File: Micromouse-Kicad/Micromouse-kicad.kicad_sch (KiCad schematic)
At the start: 101 parts, among them J1 SWD, J2 USB_B_Micro, J3 UARTBTH, J4 Batería, J5 VL6180x, J6 MotorEncodL, J7 MotorEncodR, Q1 BS170, Q2 BS170, Q3 BS170, Q4 BS170, SW1 RST, SW2 BootSwitch, SW3 PowerSwitch, SW4 BTN, SW5 BTN, U1 STM32F405RGT6, U10 TCRT5000, U2 AMS1117-5.0, U3 AMS1117-3.3, U4 SRV05-4, U5 MPU-6500, U6 DRV8833PWPR, U7 TCRT5000, U8 TCRT5000, U9 TCRT5000, Y1 8MHz

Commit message: Casi todo routeado
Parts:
- R4: footprint Resistor_SMD:R_0402_1005Metric -> Resistor_SMD:R_0603_1608Metric
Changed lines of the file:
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@@
       (effects (font (size 1.27 1.27)) (justify left))
     )
-    (property "Footprint" "Resistor_SMD:R_0402_1005Metric" (id 2) (at 165.1 157.48 0)
+    (property "Footprint" "Resistor_SMD:R_0603_1608Metric" (id 2) (at 165.1 157.48 0)
       (effects (font (size 1.27 1.27)) hide)
     )
@@
     )
     (path "/45c613f9-aec8-424a-b480-e2cd3c7f1c41"
-      (reference "R4") (unit 1) (value "220") (footprint "Resistor_SMD:R_0402_1005Metric")
+      (reference "R4") (unit 1) (value "220") (footprint "Resistor_SMD:R_0603_1608Metric")
     )
     (path "/3e5cccc0-5e8e-4d7a-84ba-3564961b6bdd"

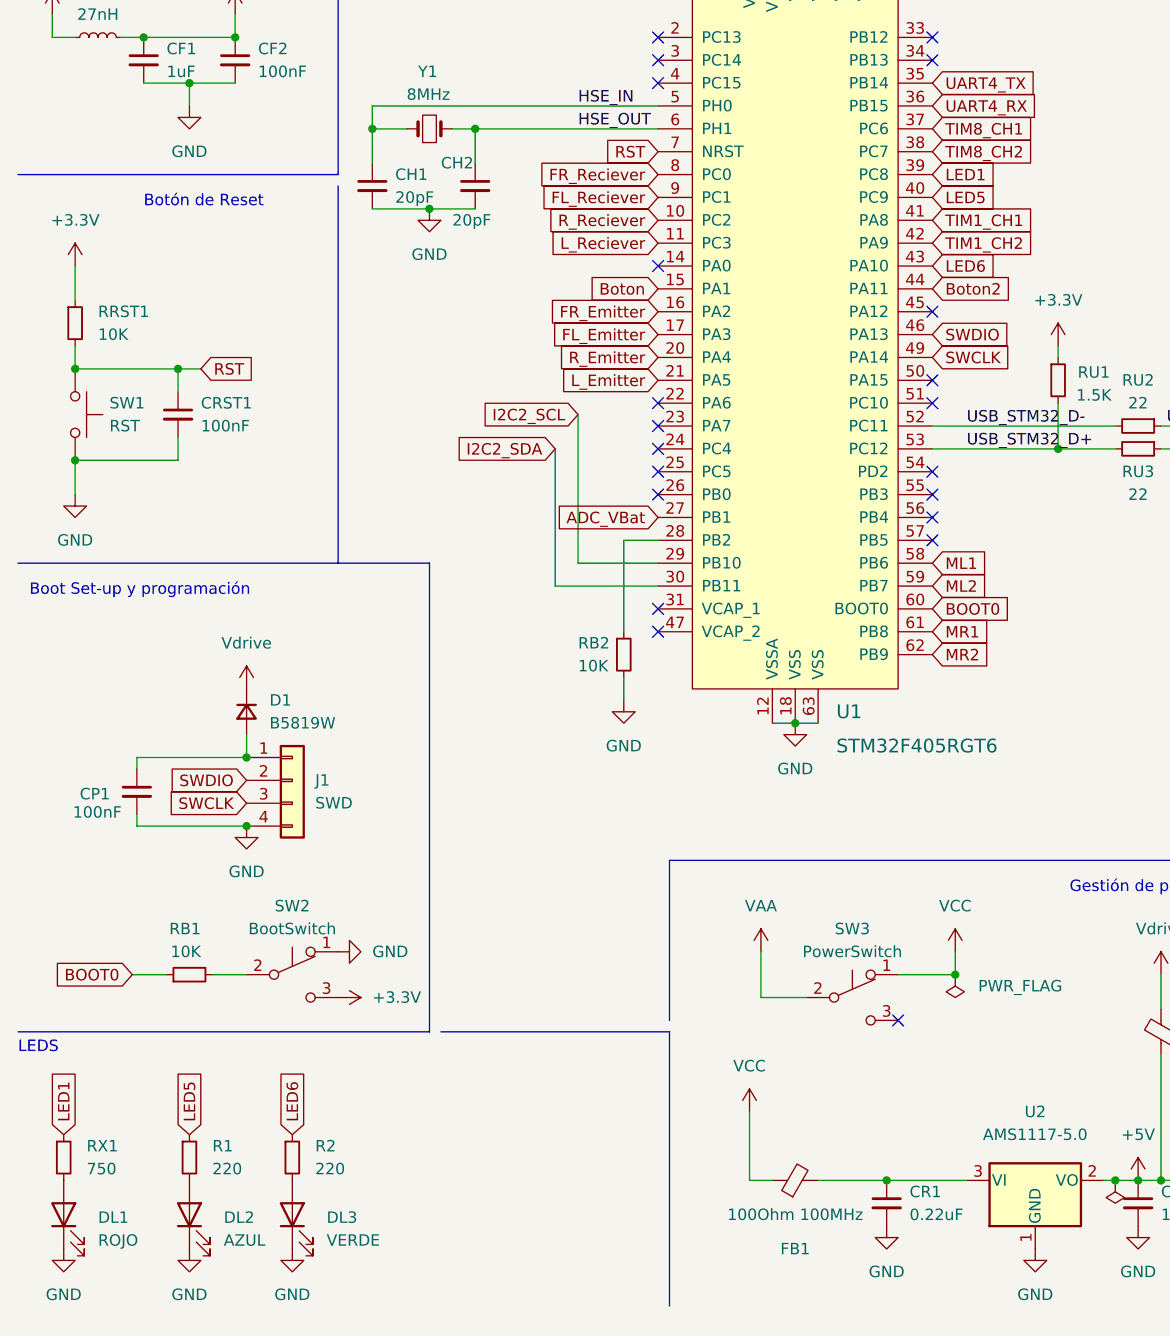
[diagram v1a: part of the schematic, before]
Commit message: PCB Completa - Depurada
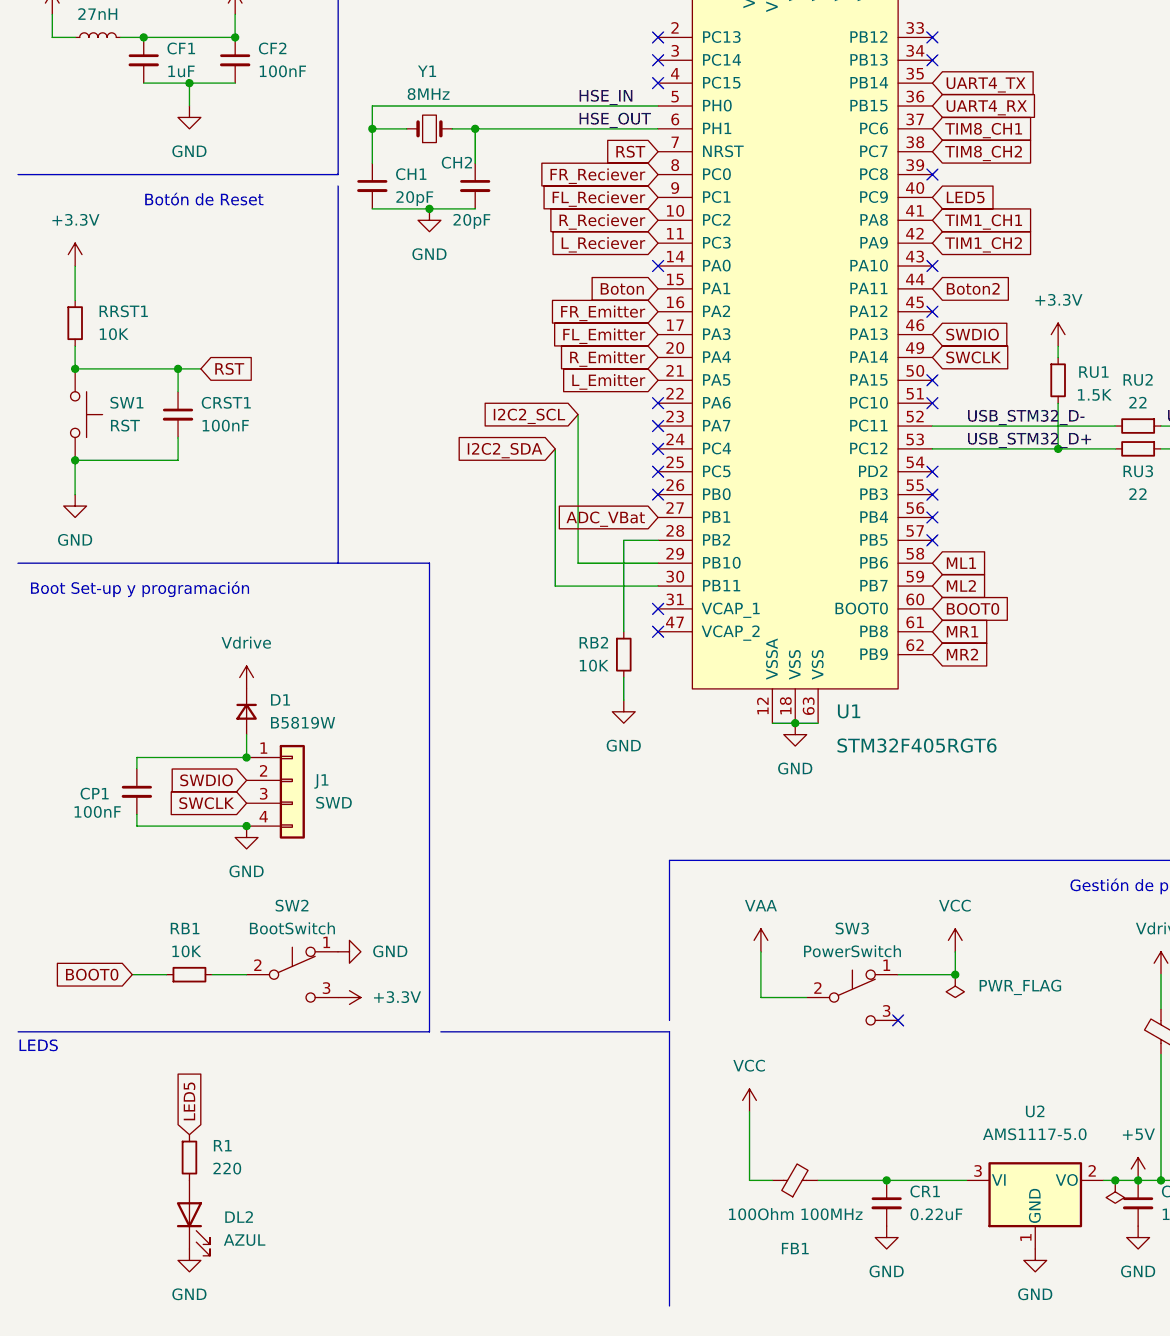
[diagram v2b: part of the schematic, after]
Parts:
- removed DL1: ROJO, LED_SMD:LED_0603_1608Metric, symbol Device:LED
- removed DL3: VERDE, LED_SMD:LED_0603_1608Metric, symbol Device:LED
- removed R2: 220, Resistor_SMD:R_0603_1608Metric, symbol Device:R_Small
- removed RX1: 750, Resistor_SMD:R_0603_1608Metric, symbol Device:R_Small
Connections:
- net LED1: no longer names the net of U1.39 (PC8)
- net LED6: no longer names the net of U1.43 (PA10)
- no-connect marks 37 -> 39
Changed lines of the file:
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@@
   (no_connect (at 200.66 49.53))
   (no_connect (at 200.66 36.83))
+  (no_connect (at 114.3 81.28))
+  (no_connect (at 114.3 71.12))
   (no_connect (at 256.54 92.71))
   (no_connect (at 154.94 96.52))
@@
     )
   )
-  (global_label "LED6" (shape input) (at 114.3 81.28 0) (fields_autoplaced)
-    (effects (font (size 1.27 1.27)) (justify left))
-    (property "Intersheet References" "${INTERSHEET_REFS}" (id 0) (at 121.3698 81.2006 0)
-      (effects (font (size 1.27 1.27)) (justify left) hide)
-    )
-  )
   (global_label "Boton" (shape input) (at 83.82 83.82 180) (fields_autoplaced)
     (effects (font (size 1.27 1.27)) (justify right))
@@
     )
   )
-  (global_label "LED1" (shape input) (at 114.3 71.12 0) (fields_autoplaced)
-    (effects (font (size 1.27 1.27)) (justify left))
-    (property "Intersheet References" "${INTERSHEET_REFS}" (id 0) (at 121.3698 71.0406 0)
-      (effects (font (size 1.27 1.27)) (justify left) hide)
-    )
-  )
   (global_label "SWDIO" (shape input) (at 38.1 138.43 180) (fields_autoplaced)
     (effects (font (size 1.27 1.27)) (justify right))
@@
     )
   )
-  (global_label "LED1" (shape input) (at 17.78 177.8 90) (fields_autoplaced)
-    (effects (font (size 1.27 1.27)) (justify left))
-    (property "Intersheet References" "${INTERSHEET_REFS}" (id 0) (at 17.7006 170.7302 90)
-      (effects (font (size 1.27 1.27)) (justify left) hide)
-    )
-  )
   (global_label "OutML1" (shape input) (at 271.78 73.66 0) (fields_autoplaced)
     (effects (font (size 1.27 1.27)) (justify left))
@@
     )
   )
-  (global_label "LED6" (shape input) (at 43.18 177.8 90) (fields_autoplaced)
-    (effects (font (size 1.27 1.27)) (justify left))
-    (property "Intersheet References" "${INTERSHEET_REFS}" (id 0) (at 43.1006 170.7302 90)
-      (effects (font (size 1.27 1.27)) (justify left) hide)
-    )
-  )
   (global_label "I2C2_SCL" (shape input) (at 74.93 97.79 180) (fields_autoplaced)
     (effects (font (size 1.27 1.27)) (justify right))
@@
     (pin "2")
   )
-  (symbol (lib_id "power:GND") (at 43.18 190.5 0) (unit 1)
-    (in_bom yes) (on_board yes) (fields_autoplaced)
-    (property "Reference" "#PWR012" (id 0) (at 43.18 196.85 0)
-      (effects (font (size 1.27 1.27)) hide)
-    )
-    (property "Value" "GND" (id 1) (at 43.18 195.58 0))
-    (property "Footprint" "" (id 2) (at 43.18 190.5 0)
-      (effects (font (size 1.27 1.27)) hide)
-    )
-    (property "Datasheet" "" (id 3) (at 43.18 190.5 0)
-      (effects (font (size 1.27 1.27)) hide)
-    )
-    (pin "1")
-  )
   (symbol (lib_id "power:GND") (at 149.86 190.5 0) (unit 1)
     (in_bom yes) (on_board yes) (fields_autoplaced)
@@
     (pin "2")
   )
-  (symbol (lib_id "Device:LED") (at 43.18 186.69 90) (unit 1)
-    (in_bom yes) (on_board yes)
-    (property "Reference" "DL3" (id 0) (at 46.99 187.0074 90)
-      (effects (font (size 1.27 1.27)) (justify right))
-    )
-    (property "Value" "VERDE" (id 1) (at 46.99 189.5474 90)
-      (effects (font (size 1.27 1.27)) (justify right))
-    )
-    (property "Footprint" "LED_SMD:LED_0603_1608Metric" (id 2) (at 43.18 186.69 0)
-      (effects (font (size 1.27 1.27)) hide)
-    )
-    (property "Datasheet" "~" (id 3) (at 43.18 186.69 0)
-      (effects (font (size 1.27 1.27)) hide)
-    )
-    (pin "1")
-    (pin "2")
-  )
   (symbol (lib_id "Device:C_Small") (at 16.51 27.94 0) (unit 1)
     (in_bom yes) (on_board yes) (fields_autoplaced)
@@
     (pin "9")
   )
-  (symbol (lib_id "Device:R_Small") (at 43.18 180.34 0) (unit 1)
-    (in_bom yes) (on_board yes) (fields_autoplaced)
-    (property "Reference" "R2" (id 0) (at 45.72 179.0699 0)
-      (effects (font (size 1.27 1.27)) (justify left))
-    )
-    (property "Value" "220" (id 1) (at 45.72 181.6099 0)
-      (effects (font (size 1.27 1.27)) (justify left))
-    )
-    (property "Footprint" "Resistor_SMD:R_0603_1608Metric" (id 2) (at 43.18 180.34 0)
-      (effects (font (size 1.27 1.27)) hide)
-    )
-    (property "Datasheet" "~" (id 3) (at 43.18 180.34 0)
-      (effects (font (size 1.27 1.27)) hide)
-    )
-    (pin "1")
-    (pin "2")
-  )
   (symbol (lib_id "power:+3.3V") (at 260.35 119.38 0) (unit 1)
     (in_bom yes) (on_board yes) (fields_autoplaced)
@@
     (pin "2")
   )
-  (symbol (lib_id "Device:R_Small") (at 17.78 180.34 0) (unit 1)
-    (in_bom yes) (on_board yes) (fields_autoplaced)
-    (property "Reference" "RX1" (id 0) (at 20.32 179.0699 0)
-      (effects (font (size 1.27 1.27)) (justify left))
-    )
-    (property "Value" "750" (id 1) (at 20.32 181.6099 0)
-      (effects (font (size 1.27 1.27)) (justify left))
-    )
-    (property "Footprint" "Resistor_SMD:R_0603_1608Metric" (id 2) (at 17.78 180.34 0)
-      (effects (font (size 1.27 1.27)) hide)
-    )
-    (property "Datasheet" "~" (id 3) (at 17.78 180.34 0)
-      (effects (font (size 1.27 1.27)) hide)
-    )
-    (pin "1")
-    (pin "2")
-  )
   (symbol (lib_id "power:GND") (at 285.75 170.18 270) (unit 1)
     (in_bom yes) (on_board yes) (fields_autoplaced)
@@
     (pin "1")
   )
-  (symbol (lib_id "power:GND") (at 17.78 190.5 0) (unit 1)
-    (in_bom yes) (on_board yes) (fields_autoplaced)
-    (property "Reference" "#PWR02" (id 0) (at 17.78 196.85 0)
-      (effects (font (size 1.27 1.27)) hide)
-    )
-    (property "Value" "GND" (id 1) (at 17.78 195.58 0))
-    (property "Footprint" "" (id 2) (at 17.78 190.5 0)
-      (effects (font (size 1.27 1.27)) hide)
-    )
-    (property "Datasheet" "" (id 3) (at 17.78 190.5 0)
-      (effects (font (size 1.27 1.27)) hide)
-    )
-    (pin "1")
-  )
   (symbol (lib_id "power:VAA") (at 209.55 173.99 270) (unit 1)
     (in_bom yes) (on_board yes) (fields_autoplaced)
@@
     (pin "1")
   )
-  (symbol (lib_id "Device:LED") (at 17.78 186.69 90) (unit 1)
-    (in_bom yes) (on_board yes) (fields_autoplaced)
-    (property "Reference" "DL1" (id 0) (at 21.59 187.0074 90)
-      (effects (font (size 1.27 1.27)) (justify right))
-    )
-    (property "Value" "ROJO" (id 1) (at 21.59 189.5474 90)
-      (effects (font (size 1.27 1.27)) (justify right))
-    )
-    (property "Footprint" "LED_SMD:LED_0603_1608Metric" (id 2) (at 17.78 186.69 0)
-      (effects (font (size 1.27 1.27)) hide)
-    )
-    (property "Datasheet" "~" (id 3) (at 17.78 186.69 0)
-      (effects (font (size 1.27 1.27)) hide)
-    )
-    (pin "1")
-    (pin "2")
-  )
   (symbol (lib_id "power:+3.3V") (at 410.21 85.09 0) (unit 1)
     (in_bom yes) (on_board yes) (fields_autoplaced)
@@
       (reference "#PWR01") (unit 1) (value "+3.3V") (footprint "")
     )
-    (path "/be344b93-f0c0-489b-b68e-ea1eb4ebd301"
-      (reference "#PWR02") (unit 1) (value "GND") (footprint "")
-    )
     (path "/8d533f32-19b8-4d37-9b18-85480ab04d92"
       (reference "#PWR03") (unit 1) (value "+3.3V") (footprint "")
@@
       (reference "#PWR011") (unit 1) (value "GND") (footprint "")
     )
-    (path "/09b16a4c-98eb-4a63-a90c-d7792ed4bea8"
-      (reference "#PWR012") (unit 1) (value "GND") (footprint "")
-    )
     (path "/e1aec55e-33df-471e-82f8-1ffd557fcb18"
       (reference "#PWR013") (unit 1) (value "GND") (footprint "")
@@
       (reference "D2") (unit 1) (value "B5819W") (footprint "Diode_SMD:D_SOD-123")
     )
-    (path "/e6712806-8c22-44f2-bf7d-4a2d10fe6d5c"
-      (reference "DL1") (unit 1) (value "ROJO") (footprint "LED_SMD:LED_0603_1608Metric")
-    )
     (path "/7134e756-0a61-443f-bb6d-fecdd623881a"
       (reference "DL2") (unit 1) (value "AZUL") (footprint "LED_SMD:LED_0603_1608Metric")
     )
-    (path "/4600a087-6880-437d-af91-1e84be1a1d53"
-      (reference "DL3") (unit 1) (value "VERDE") (footprint "LED_SMD:LED_0603_1608Metric")
-    )
     (path "/5fbf1597-61af-4c6c-89a9-660ed6185769"
       (reference "DL7") (unit 1) (value "VERDE") (footprint "LED_SMD:LED_0603_1608Metric")
@@
       (reference "R1") (unit 1) (value "220") (footprint "Resistor_SMD:R_0603_1608Metric")
     )
-    (path "/86c5061d-8e09-4bab-b0e5-86f6707d9e5e"
-      (reference "R2") (unit 1) (value "220") (footprint "Resistor_SMD:R_0603_1608Metric")
-    )
     (path "/45c613f9-aec8-424a-b480-e2cd3c7f1c41"
       (reference "R4") (unit 1) (value "220") (footprint "Resistor_SMD:R_0603_1608Metric")
@@
       (reference "RU3") (unit 1) (value "22") (footprint "Resistor_SMD:R_0603_1608Metric")
     )
-    (path "/a5ccd16c-0207-46ed-a536-7bf8b96e3f2b"
-      (reference "RX1") (unit 1) (value "750") (footprint "Resistor_SMD:R_0603_1608Metric")
-    )
     (path "/904ae360-b03d-4f3f-a237-22e33f2af105"

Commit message: Modelo 3D
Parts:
- J6, J7: footprint Connector_JST:JST_XH_B6B-XH-A_1x06_P2.50mm_Vertical -> Connector_JST:JST_SHL_SM06B-SHLS-TF_1x06-1MP_P1.00mm_Horizontal
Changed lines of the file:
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@@
       (effects (font (size 1.27 1.27)) (justify left))
     )
-    (property "Footprint" "Connector_JST:JST_XH_B6B-XH-A_1x06_P2.50mm_Vertical" (id 2) (at 290.83 175.26 0)
+    (property "Footprint" "Connector_JST:JST_SHL_SM06B-SHLS-TF_1x06-1MP_P1.00mm_Horizontal" (id 2) (at 290.83 175.26 0)
       (effects (font (size 1.27 1.27)) hide)
     )
@@
       (effects (font (size 1.27 1.27)) (justify left))
     )
-    (property "Footprint" "Connector_JST:JST_XH_B6B-XH-A_1x06_P2.50mm_Vertical" (id 2) (at 256.54 175.26 0)
+    (property "Footprint" "Connector_JST:JST_SHL_SM06B-SHLS-TF_1x06-1MP_P1.00mm_Horizontal" (id 2) (at 256.54 175.26 0)
       (effects (font (size 1.27 1.27)) hide)
     )
@@
     )
     (path "/6b173ad2-a80e-42b7-b9a4-03e34411ed68"
-      (reference "J6") (unit 1) (value "MotorEncodL") (footprint "Connector_JST:JST_XH_B6B-XH-A_1x06_P2.50mm_Vertical")
+      (reference "J6") (unit 1) (value "MotorEncodL") (footprint "Connector_JST:JST_SHL_SM06B-SHLS-TF_1x06-1MP_P1.00mm_Horizontal")
     )
     (path "/2301f17e-45ec-4ade-8b9e-4d97bea85791"
-      (reference "J7") (unit 1) (value "MotorEncodR") (footprint "Connector_JST:JST_XH_B6B-XH-A_1x06_P2.50mm_Vertical")
+      (reference "J7") (unit 1) (value "MotorEncodR") (footprint "Connector_JST:JST_SHL_SM06B-SHLS-TF_1x06-1MP_P1.00mm_Horizontal")
     )
     (path "/3263ba06-1178-4ee5-967f-6cb2162e5cc6"
